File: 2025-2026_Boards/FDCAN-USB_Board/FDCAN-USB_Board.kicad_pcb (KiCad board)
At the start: 2 copper layers, 39 x 34 mm, 53 parts, among them J1 USB4110GFA, J2 Conn_01x03_Socket, J3 Conn_01x03_Socket, J4 Conn_01x02_Pin, J5 Conn_01x02_Pin, J6 Conn_ARM_JTAG_SWD_10, U1 AMS1117-3.3, U2 USBLC6-2SC6, U3 STM32G474CETx, U4 TCAN1057AEV-Q1, U5 TCAN1057AEV-Q1

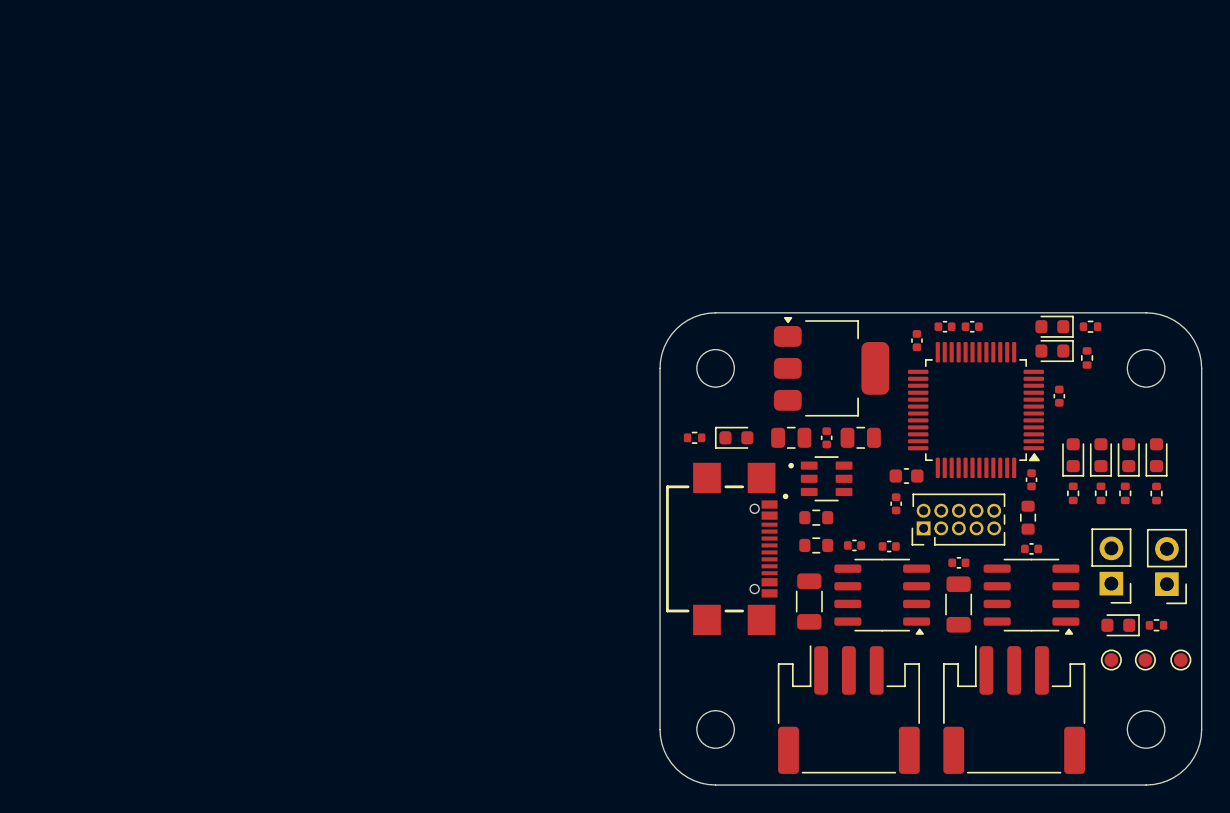
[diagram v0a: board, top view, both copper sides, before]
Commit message: Layout finished
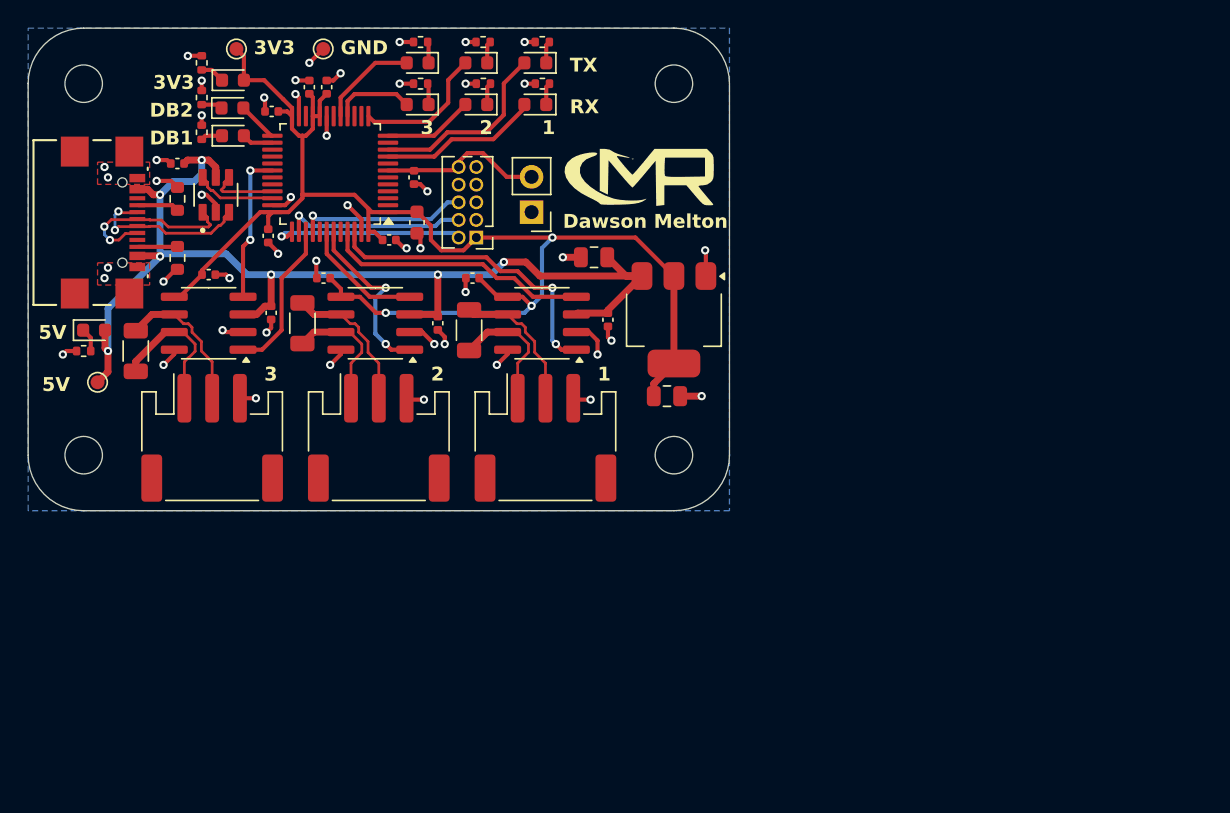
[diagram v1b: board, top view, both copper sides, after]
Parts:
- removed J1: USB4110GFA, Cornell_Mars_Rover:GCT_USB4110GFA
- added C13: 1u, Capacitor_SMD:C_0402_1005Metric, F.Cu at (92.5, 70.5)
- added C14: 1u, Capacitor_SMD:C_0402_1005Metric, F.Cu at (96.3, 68.0)
- added D5: GREEN, LED_SMD:LED_0603_1608Metric, F.Cu at (103.0, 52.5)
- added D8: YELLOW, LED_SMD:LED_0603_1608Metric, F.Cu at (103.0, 55.5)
- added G***: LOGO, Cornell_Mars_Rover:CMR_Logo, F.Cu at (119.0, 61.8)
- added J7: USB4110-GF-A, Cornell_Mars_Rover:USB4110-GF-A_GCT, F.Cu at (79.5, 64.0)
- added R14: 1k, Resistor_SMD:R_0402_1005Metric, F.Cu at (103.3, 51.0)
- added R15: 1k, Resistor_SMD:R_0402_1005Metric, F.Cu at (103.3, 54.0)
- added U6: TCAN1057AEV-Q1, Package_SO:SOIC-8_3.9x4.9mm_P1.27mm, F.Cu at (88.0, 71.2)
- D10: renamed from D8; value YELLOW -> BLUE
- D6: renamed from D4; value GREEN -> YELLOW
- D7: renamed from D6; value GREEN -> YELLOW
- D9: renamed from D7; value YELLOW -> BLUE
- J4: value Conn_01x02_Pin -> Conn_01x03_Socket; footprint Connector_PinHeader_2.54mm:PinHeader_1x02_P2.54mm_Vertical -> Connector_JST:JST_PH_S3B-PH-SM4-TB_1x03-1MP_P2.00mm_Horizontal
- R13: value 10k -> 120; footprint Resistor_SMD:R_0603_1608Metric -> Resistor_SMD:R_1206_3216Metric
- moved R6 79.8 mm to (87.5, 52.5), turned to 90 degrees
- moved TP2 78.9 mm to (90.0, 51.5)
- moved TP1 75.8 mm to (96.2, 51.5), turned to 180 degrees
- moved TP3 75.7 mm to (80.0, 75.5)
- moved D2 74.9 mm to (89.8, 53.8), turned to 0 degrees
- moved R8 74.4 mm to (87.5, 55.0), turned to 90 degrees
- moved R7 71.4 mm to (87.5, 57.5), turned to 90 degrees
- moved D10 71.1 mm to (89.7, 55.8), turned to 0 degrees
- moved D9 68.5 mm to (89.7, 57.8), turned to 0 degrees
- moved J4 65.6 mm to (88.2, 79.5), turned to 0 degrees
- moved R13 65.4 mm to (82.8, 73.2), turned to 90 degrees
- moved C4 57.9 mm to (88.0, 67.8), turned to 0 degrees
- moved J5 53.0 mm to (111.2, 63.2)
- moved R9 51.7 mm to (112.0, 51.0), turned to 180 degrees
- moved R2 51.4 mm to (85.8, 62.3), turned to -90 degrees
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- renumbered D5 to D4
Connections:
- net CANH1 renamed CAN1+
- net CANH2 renamed CAN2+
- net CANL1 renamed CAN1-
- net CANL2 renamed CAN2-
- net USB_DM renamed USB_N
- net USB_DP renamed USB_P
- J4 pad 1: 3.3V -> CAN3+
- J4 pad 2: BOOT0 -> CAN3-
- R1 pad 1: Net-(J1-CC2) -> GND
- R1 pad 2: GND -> Net-(J7-CC2)
- R13 pad 1: BOOT0 -> CAN3+
- R13 pad 2: GND -> CAN3-
- R2 pad 1: Net-(J1-CC1) -> GND
- R2 pad 2: GND -> Net-(J7-CC1)
- U3 pad 10: LED_RX_1 -> LED_TX_1
- U3 pad 12: LED_TX_1 -> LED_RX_2
- U3 pad 13: unconnected-(U3-PA5-Pad13) -> LED_TX_2
- U3 pad 14: LED_RX_2 -> unconnected-(U3-PA6-Pad14)
- U3 pad 16: LED_TX_2 -> LED_RX_3
- U3 pad 17: unconnected-(U3-PB1-Pad17) -> LED_TX_3
- U3 pad 2: LED_Debug1 -> unconnected-(U3-PC13-Pad2)
- U3 pad 25: unconnected-(U3-PB11-Pad25) -> LED_Debug2
- U3 pad 26: CAN_RX1 -> LED_Debug1
- U3 pad 27: CAN_TX1 -> unconnected-(U3-PB13-Pad27)
- U3 pad 30: CAN_RX2 -> CAN_RX3
- U3 pad 39: CAN_TX2 -> CAN_TX3
- U3 pad 4: LED_Debug2 -> unconnected-(U3-PC15-Pad4)
- U3 pad 42: unconnected-(U3-PB5-Pad42) -> CAN_RX2
- U3 pad 43: unconnected-(U3-PB6-Pad43) -> CAN_TX2
- U3 pad 45: BOOT0 -> CAN_RX1
- U3 pad 46: unconnected-(U3-PB9-Pad46) -> CAN_TX1
- U3 pad 9: unconnected-(U3-PA1-Pad9) -> LED_RX_1
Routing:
- net 3.3V: track 0.00 -> 103.4 mm, vias 0 -> 3
- net 5V: track 0.00 -> 83.4 mm, vias 0 -> 7
- net GND: track 0.00 -> 56.8 mm, vias 0 -> 48
- net CAN_TX1: track 0.00 -> 22.4 mm, vias 0 -> 2
- net CAN_RX1: track 0.00 -> 19.2 mm
- net SWDIO: track 0.00 -> 13.9 mm, vias 0 -> 1
- net LED_TX_1: track 0.00 -> 13.7 mm
- net SWCLK: track 0.00 -> 13.2 mm, vias 0 -> 1
- net CAN_TX2: track 0.00 -> 12.8 mm, vias 0 -> 2
- net USB+: track 0.00 -> 12.6 mm, vias 0 -> 2
- net SWO: track 0.00 -> 12.3 mm, vias 0 -> 1
- net USB-: track 0.00 -> 12.2 mm, vias 0 -> 2
- net NRST: track 0.00 -> 11.8 mm
- net LED_RX_1: track 0.00 -> 11.5 mm
- net CAN_TX3: track 0.00 -> 11.2 mm
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- added copper zone on B.Cu, net GND
- added copper zone on F.Cu, net GND
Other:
- board size 39 x 34 mm -> 50.5 x 34.8 mm
- board text added: "1"
- board text added: "2"
- board text added: "3"
- board text added: "3V3"
- board text added: "5V"
- board text added: "DB1"
- board text added: "DB2"
- board text added: "Dawson Melton"
- board text added: "GND"
- board text added: "RX"
- board text added: "TX"
